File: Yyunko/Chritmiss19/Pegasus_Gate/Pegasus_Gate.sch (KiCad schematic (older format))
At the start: 37 parts, among them J1 Conn_01x03_Female, J2 Conn_01x03_Female, U1 WS2811, U2 WS2811, U3 WS2811, U4 1528-1537-ND

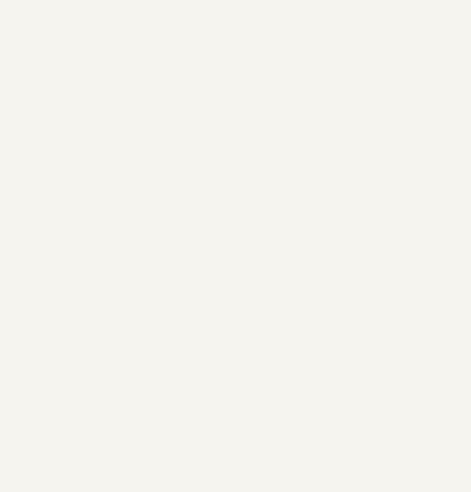
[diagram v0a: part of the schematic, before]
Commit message: Continue work on durg ring thing
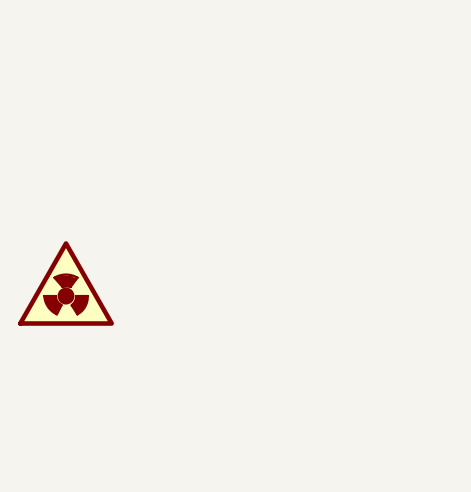
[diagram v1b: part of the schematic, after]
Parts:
- added SYM1: SYM_Radioactive_Large, Local:DragonIcon, symbol Graphic:SYM_Radioactive_Large
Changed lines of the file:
@@
 Wire Wire Line
 	10625 2225 10625 2175
+$Comp
+L Graphic:SYM_Radioactive_Large SYM1
+U 1 1 5DE0498B
+P 2700 6025
+F 0 "SYM1" H 2795 6305 50  0001 C CNN
+F 1 "SYM_Radioactive_Large" H 2795 5855 50  0001 C CNN
+F 2 "Local:DragonIcon" H 2795 5905 50  0001 C CNN
+F 3 "~" H 2825 5905 50  0001 C CNN
+	1    2700 6025
+	1    0    0    -1
+$EndComp
 $EndSCHEMATC
